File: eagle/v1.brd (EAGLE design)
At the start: 24.2 x 49.6 mm, 40 parts, among them IC2 LT1761, IC4 LT1376-ADJ, Q1 12Mhz, T1 Si2301DS, X1 USB-MICROB

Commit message: small change
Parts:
- R6: value 15k -> 680k
- R7: value 15k -> 220k
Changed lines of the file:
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@@
 </element>
 <element name="L2" library="seb" package="PIS2408" value="20µH/xxx mA" x="13" y="19.2" smashed="yes" rot="R270"/>
-<element name="R6" library="rcl" package="R0402" value="15k" x="10.4" y="23.8" smashed="yes" rot="R180">
+<element name="R6" library="rcl" package="R0402" value="680k" x="10.4" y="23.8" smashed="yes" rot="R180">
 <attribute name="NAME" x="10.565" y="24.635" size="0.8128" layer="25" font="vector" ratio="10"/>
 <attribute name="VALUE" x="11.035" y="25.705" size="1.27" layer="27" rot="R180"/>
 </element>
-<element name="R7" library="rcl" package="R0402" value="15k" x="8" y="23.8" smashed="yes">
+<element name="R7" library="rcl" package="R0402" value="220k" x="8" y="23.8" smashed="yes">
 <attribute name="NAME" x="7.165" y="22.235" size="0.8128" layer="25" font="vector" ratio="10"/>
 <attribute name="VALUE" x="7.365" y="21.895" size="1.27" layer="27"/>

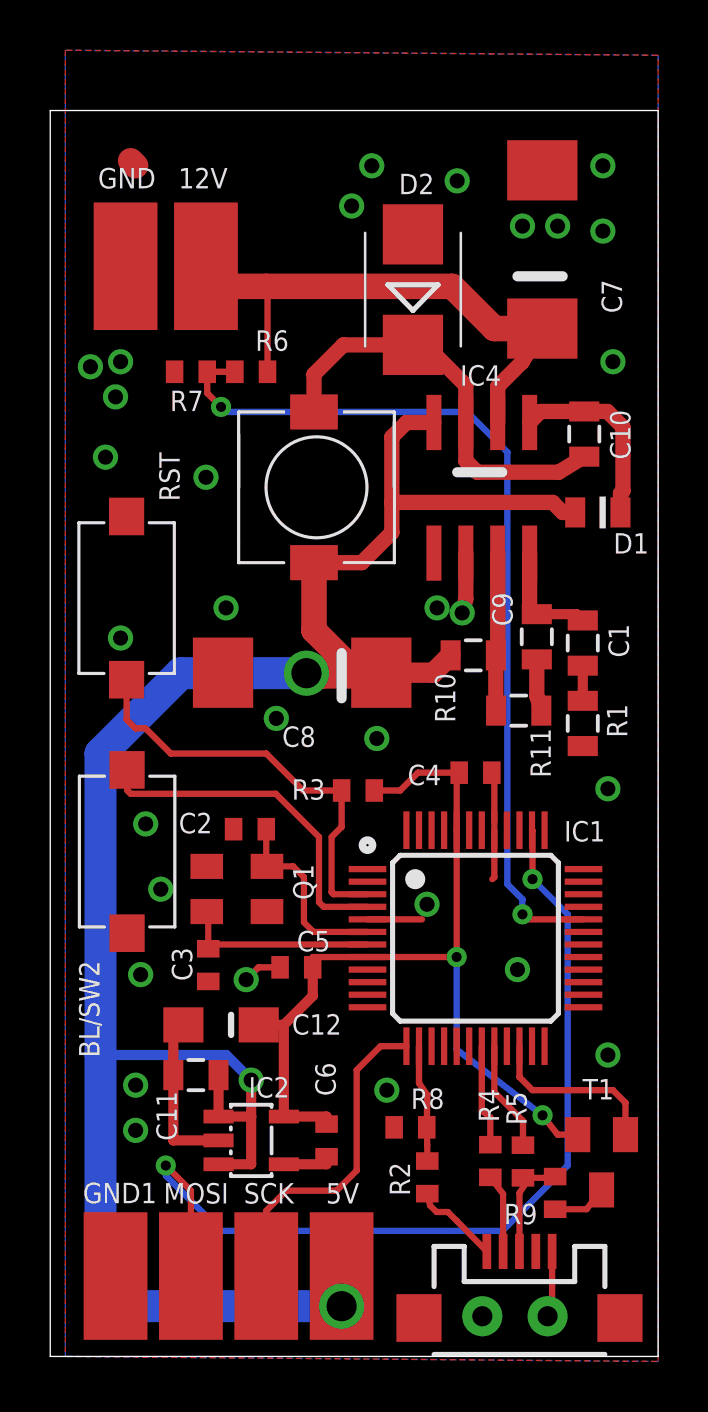
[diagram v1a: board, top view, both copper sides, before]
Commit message: i2c connector
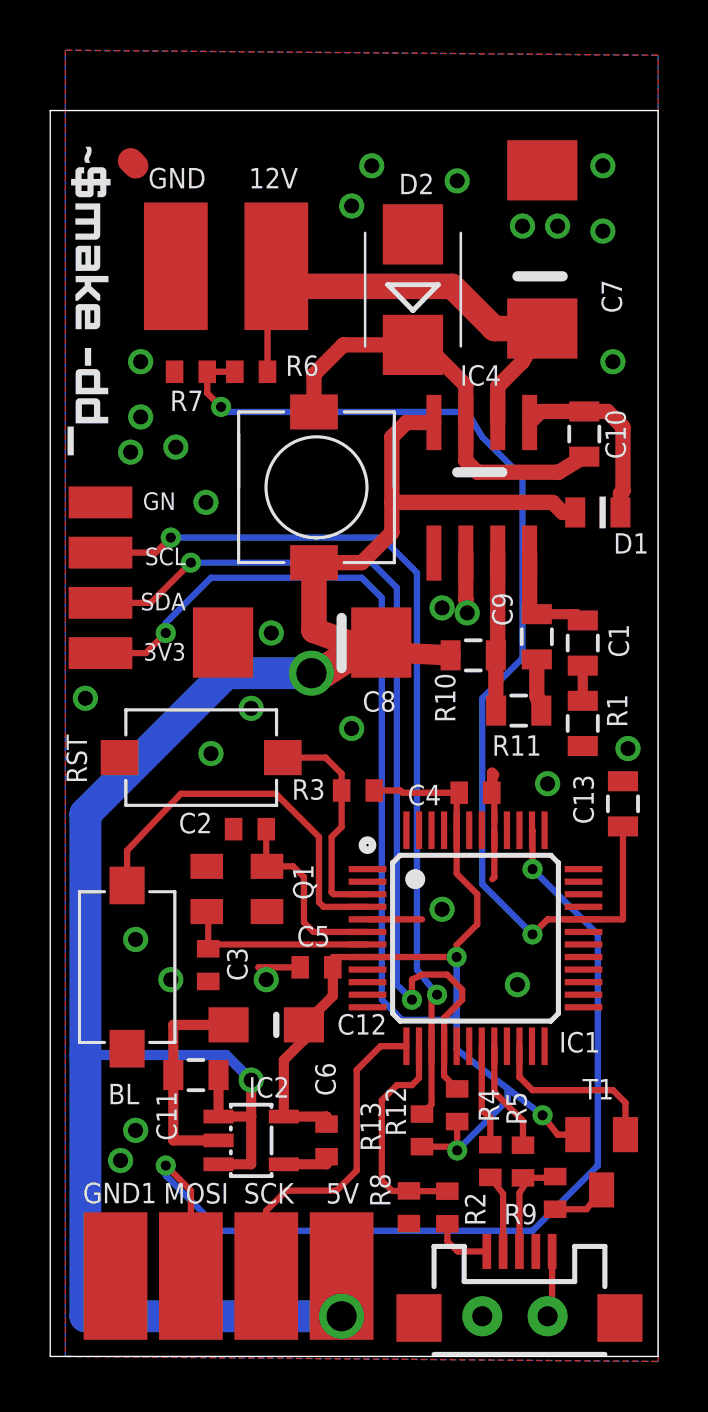
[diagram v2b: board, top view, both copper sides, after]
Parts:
- removed BL/SW2: SWITCH_MCTAEF, seb:SWITCH_MCTAEF
- added 3V3, GN, SCL, SDA: (no value), wirepad:SMD1,27-2,54
- added BL: SWITCH_MCTAEF, seb:SWITCH_MCTAEF
- added C13: 1µF, SparkFun-Capacitors:0805
- added R12, R13: 15k, rcl:R0402
- added U$1: MAKE-DD_LOGO'PROMPT', seb:MAKE-DD_LOGO_PROMPT
- moved RST 7.01 mm to (8.41, 8.44), turned to 0 degrees
- moved R8 3.18 mm to (16.7, -9.46), turned to 90 degrees
- moved 12V 2.80 mm to (11.4, 28.0)
- moved GND 2.00 mm to (7.40, 28.0)
- moved C12 1.80 mm to (11.0, -2.20)
- moved R2 1.44 mm to (18.2, -9.47)
- moved C8 1.20 mm to (12.4, 13.0)
- moved C5 0.80 mm to (13.0, 0.09)
- moved C4 0.80 mm to (19.3, 7.04)
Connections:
- new net SCL: IC1.15, R13.2, SCL.1
- new net SDA: IC1.16, R12.2, SDA.1
- net +3V3: now also 3V3.1, R12.1, R13.1
- net 01: now also BL.2; no longer BL/SW2.2
- net ADC: now also C13.1
- net GND: now also BL.1, C13.2, GN.1; no longer BL/SW2.1
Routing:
- net SDA: track 0.00 -> 37.1 mm, vias 0 -> 2
- net +3V3: track 36.3 -> 73.0 mm, vias 2 -> 4
- net SCL: track 0.00 -> 35.5 mm, vias 0 -> 2
- net RST: track 17.0 -> 8.95 mm
- net ADC: track 36.0 -> 43.3 mm
- net VBUS: track 4.67 -> 9.10 mm
- net +12V: track 24.8 -> 20.7 mm
- net GND: track 21.9 -> 25.2 mm, vias 32 -> 31
- net N$8: track 37.1 -> 38.8 mm
- net 01: track 13.8 -> 15.3 mm
- net +5V_USB: track 3.51 -> 2.43 mm
- net +5V: track 84.2 -> 85.2 mm
